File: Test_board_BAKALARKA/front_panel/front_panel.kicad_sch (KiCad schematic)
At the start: 23 parts, among them SW1 SW_Push, SW10 SW_Push, SW11 SW_Push, SW12 SW_Push, SW13 SW_Push, SW14 SW_Push, SW15 SW_Push, SW16 SW_Push, SW17 SW_Push, SW18 SW_Push, SW19 SW_Push, SW2 SW_Push, SW20 SW_Push, SW21 SW_Push, SW22 SW_Push, SW23 SW_Push, SW24 SW_Push, SW3 SW_Push, SW4 SW_Push, SW5 SW_Push, SW6 SW_Push, SW8 SW_Push, SW9 SW_Push

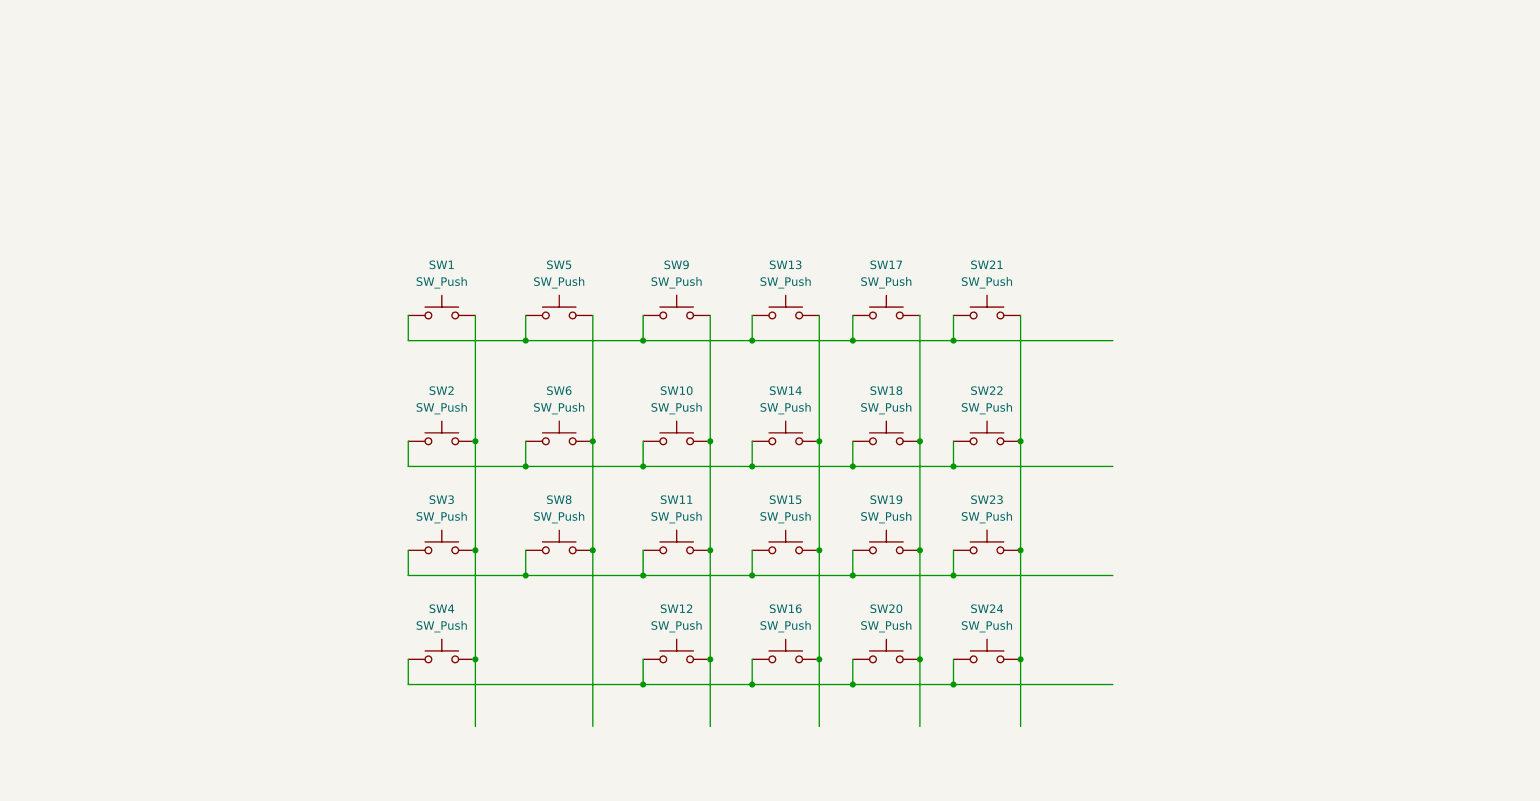
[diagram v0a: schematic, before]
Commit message: front panel and test board ordered
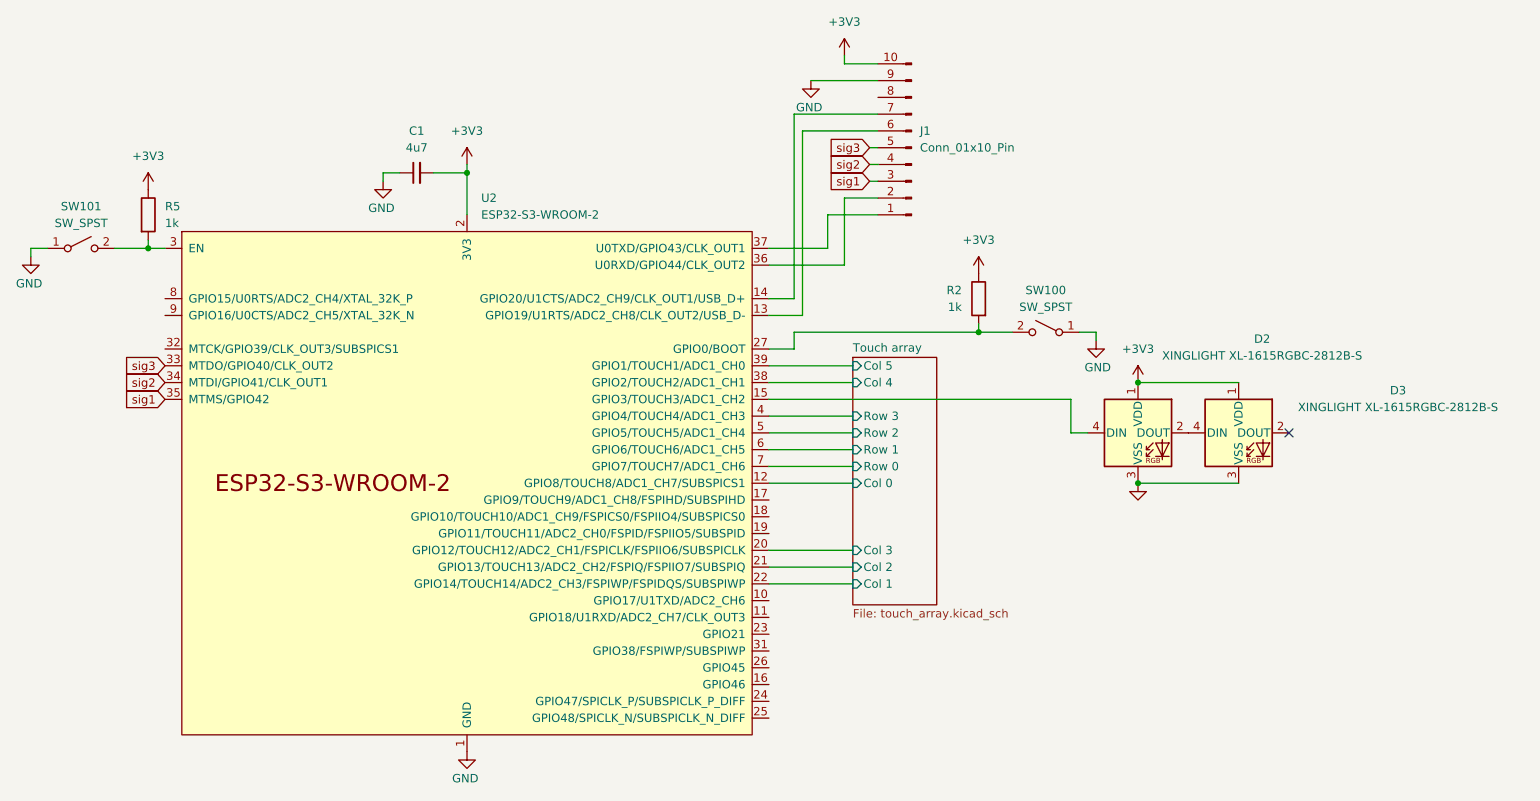
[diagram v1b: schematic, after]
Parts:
- removed SW1, SW10, SW11, SW12, SW13, SW14, SW15, SW16, SW17, SW18, SW19, SW2, SW20, SW21, SW22, SW23, SW24, SW3, SW4, SW9: SW_Push, PCM_JLCPCB:Cap_Touch_Pad, symbol Switch:SW_Push
- removed SW5, SW8: SW_Push, PCM_JLCPCB:cap_touch_triangle, symbol Switch:SW_Push
- removed SW6: SW_Push, PCM_JLCPCB:Cap_Touch_Pad_big, symbol Switch:SW_Push
- added C1: 4u7, Capacitor_SMD:C_0805_2012Metric_Pad1.18x1.45mm_HandSolder, symbol Device:C_Small
- added D2: XINGLIGHT XL-1615RGBC-2812B-S, Snapeda:XINGLIGHT XL-1615RGBC-2812B-S, symbol LED:WS2812B
- added D3: XINGLIGHT XL-1615RGBC-2812B-S, Snapeda:Flipped_XINGLIGHT XL-1615RGBC-2812B-S_1, symbol LED:WS2812B
- added J1: Conn_01x10_Pin, PCM_JLCPCB:FFC_FPC_10pin_connector, symbol Connector:Conn_01x10_Pin
- added R2, R5: 1k, Resistor_SMD:R_0603_1608Metric_Pad0.98x0.95mm_HandSolder, symbol Device:R
- added SW100, SW101: SW_SPST, Button_Switch_SMD:SW_SPST_CK_RS282G05A3, symbol Switch:SW_SPST
- added U2: ESP32-S3-WROOM-2, PCM_Espressif:ESP32-S3-WROOM-2, symbol PCM_Espressif:ESP32-S3-WROOM-2
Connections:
- new net: R2.2, SW100.2 (B), U2.27 (GPIO0/BOOT)
- new net: R5.2, SW101.2 (B), U2.3 (EN)
- new net: J1.6 (Pin_6), U2.13 (GPIO19/U1RTS/ADC2_CH8/CLK_OUT2/USB_D-)
- new net: J1.7 (Pin_7), U2.14 (GPIO20/U1CTS/ADC2_CH9/CLK_OUT1/USB_D+)
- new net: D2.4 (DIN), U2.15 (GPIO3/TOUCH3/ADC1_CH2)
- new net: J1.2 (Pin_2), U2.36 (U0RXD/GPIO44/CLK_OUT2)
- new net: J1.1 (Pin_1), U2.37 (U0TXD/GPIO43/CLK_OUT1)
- new net: D2.2 (DOUT), D3.4 (DIN)
- new net +3V3: C1.2, D2.1 (VDD), D3.1 (VDD), J1.10 (Pin_10), R2.1, R5.1, U2.2 (3V3)
- new net GND: C1.1, D2.3 (VSS), D3.3 (VSS), J1.9 (Pin_9), SW100.1 (A), SW101.1 (A), U2.1 (GND), U2.40 (GND), U2.41 (GND)
- new net Touch array/Col 0: U2.12 (GPIO8/TOUCH8/ADC1_CH7/SUBSPICS1)
- new net Touch array/Col 1: U2.22 (GPIO14/TOUCH14/ADC2_CH3/FSPIWP/FSPIDQS/SUBSPIWP)
- new net Touch array/Col 2: U2.21 (GPIO13/TOUCH13/ADC2_CH2/FSPIQ/FSPIIO7/SUBSPIQ)
- new net Touch array/Col 3: U2.20 (GPIO12/TOUCH12/ADC2_CH1/FSPICLK/FSPIIO6/SUBSPICLK)
- new net Touch array/Col 4: U2.38 (GPIO2/TOUCH2/ADC1_CH1)
- new net Touch array/Col 5: U2.39 (GPIO1/TOUCH1/ADC1_CH0)
- new net Touch array/Row 0: U2.7 (GPIO7/TOUCH7/ADC1_CH6)
- new net Touch array/Row 1: U2.6 (GPIO6/TOUCH6/ADC1_CH5)
- new net Touch array/Row 2: U2.5 (GPIO5/TOUCH5/ADC1_CH4)
- new net Touch array/Row 3: U2.4 (GPIO4/TOUCH4/ADC1_CH3)
- new net sig1: J1.3 (Pin_3), U2.35 (MTMS/GPIO42)
- new net sig2: J1.4 (Pin_4), U2.34 (MTDI/GPIO41/CLK_OUT1)
- new net sig3: J1.5 (Pin_5), U2.33 (MTDO/GPIO40/CLK_OUT2)
- no-connect marks 0 -> 1
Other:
- added sheet Touch array (touch_array.kicad_sch)
